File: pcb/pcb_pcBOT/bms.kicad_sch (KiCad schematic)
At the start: 28 parts, among them J201 Lipo, J202 USB_C_Receptacle_USB2.0_16P, SW201 ~{QON}_BUTTON, U201 BQ25896RTW

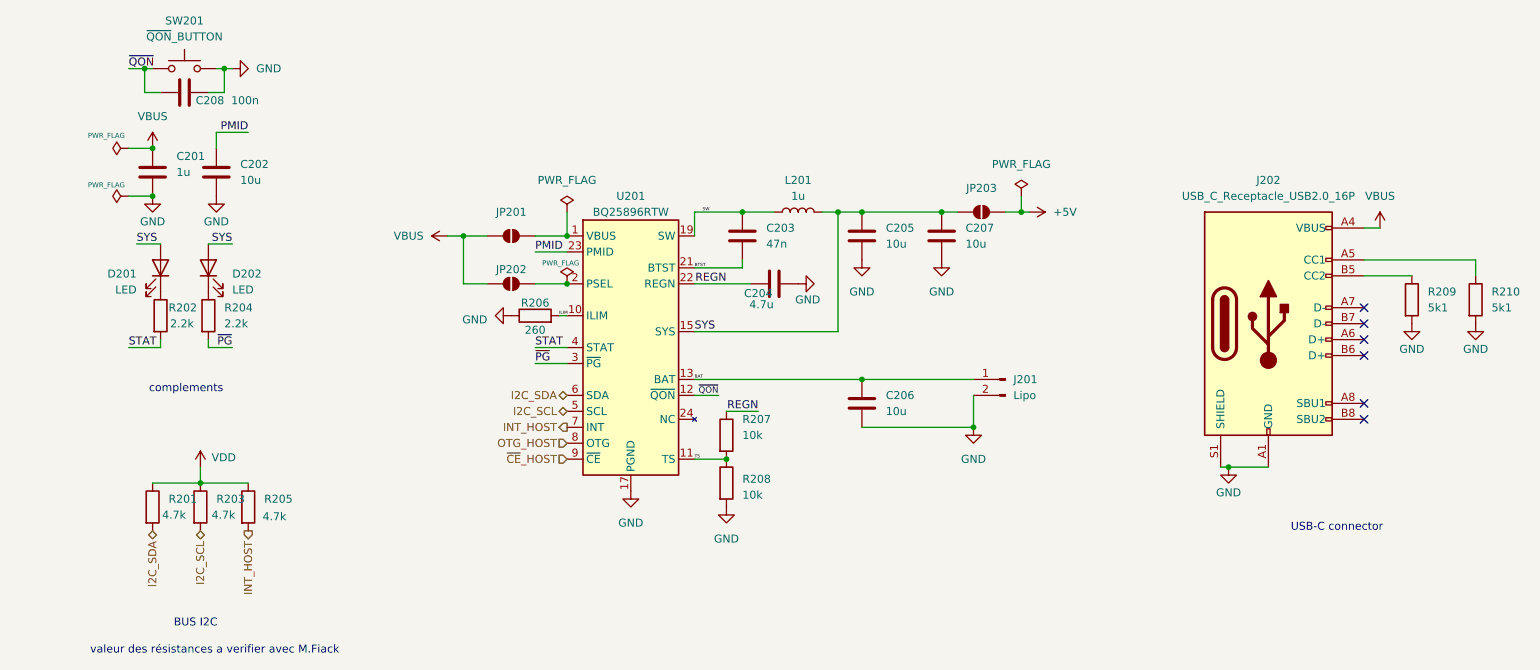
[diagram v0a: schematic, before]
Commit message: fin de schematique
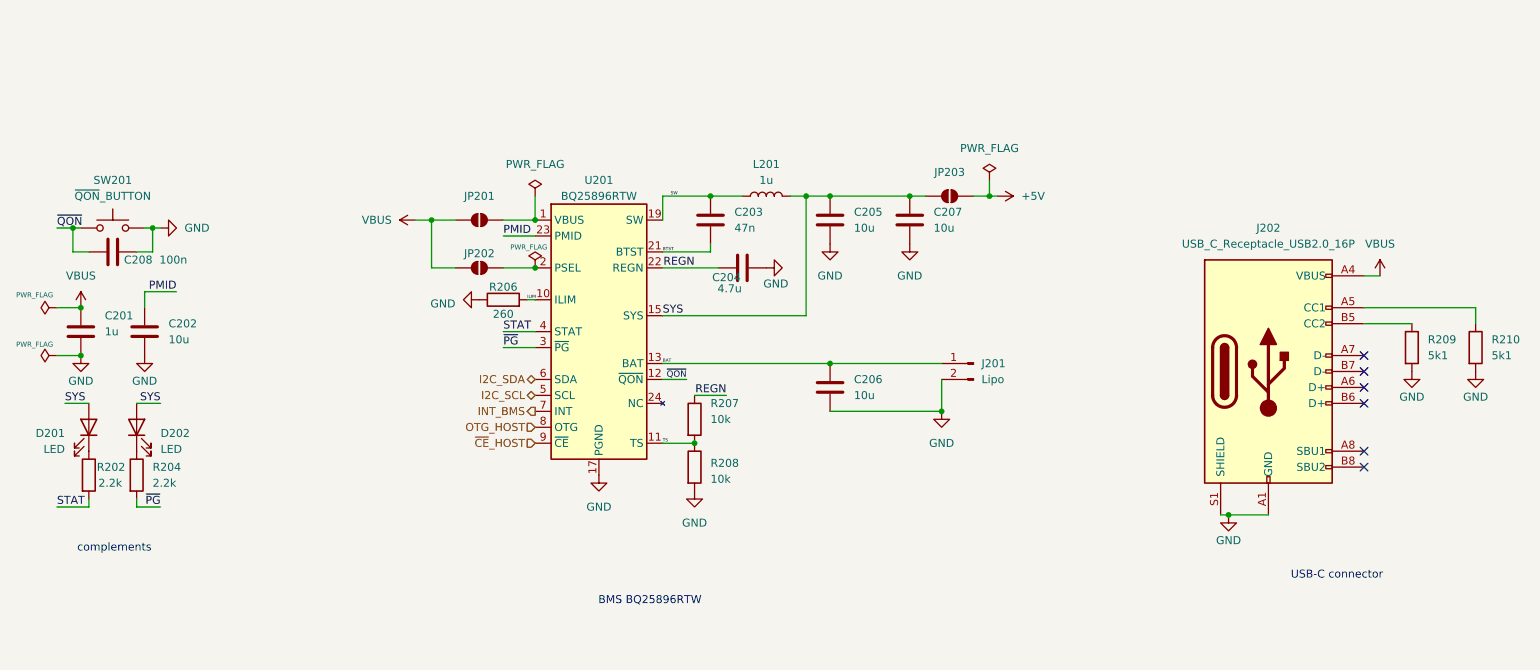
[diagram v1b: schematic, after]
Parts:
- removed R201, R203, R205: 4.7k, Resistor_SMD:R_0805_2012Metric_Pad1.20x1.40mm_HandSolder, symbol Device:R
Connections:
- net INT_HOST renamed INT_BMS
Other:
- note added: "BMS BQ25896RTW"
- note removed: "BUS I2C"
- note removed: "valeur des résistances a verifier avec M.Fiack"
- moved on the sheet: C201, C202, C203, C204, C205, C206, C207, C208, D201, D202, J201, J202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
